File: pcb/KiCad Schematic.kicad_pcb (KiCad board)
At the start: 2 copper layers, 50.1 x 70 mm, 98 parts, among them IC1 AP63205WU-7, IC2 ATSAMD51J19A-MU, J1 47571-0001, J10 Conn_01x04, J11 Conn_01x04, J12 Conn_01x03, J13 Conn_01x03, J14 Conn_01x20, J15 Conn_01x03, J16 Conn_01x03, J17 Hole, J18 Hole, J19 Hole, J2 Conn_01x02, J20 Hole, J21 Conn_01x02, J22 Conn_01x06, J3 47346-0001, J4 Conn_01x04, J5 Conn_01x04, J6 20021121-00010C4LF, J7 Conn_01x02, J8 Conn_01x02, J9 Conn_01x02, Q1 NVTFS5C680NLTAG, Q2 NVTFS5C680NLTAG, U1 TMC2041-LA, U2 TMC2041-LA, U3 AP2112K-3.3, Y1 LFXTAL009678REEL

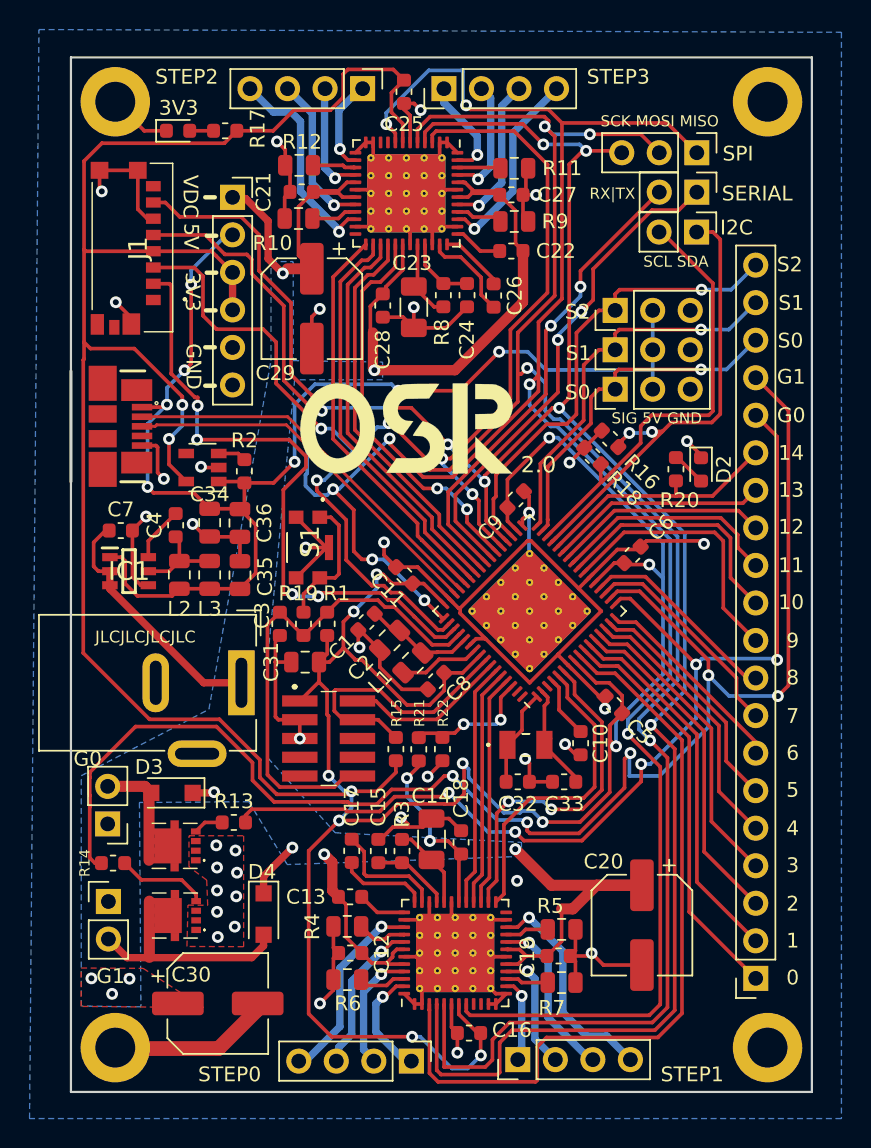
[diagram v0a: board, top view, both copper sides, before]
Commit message: arduino version bump
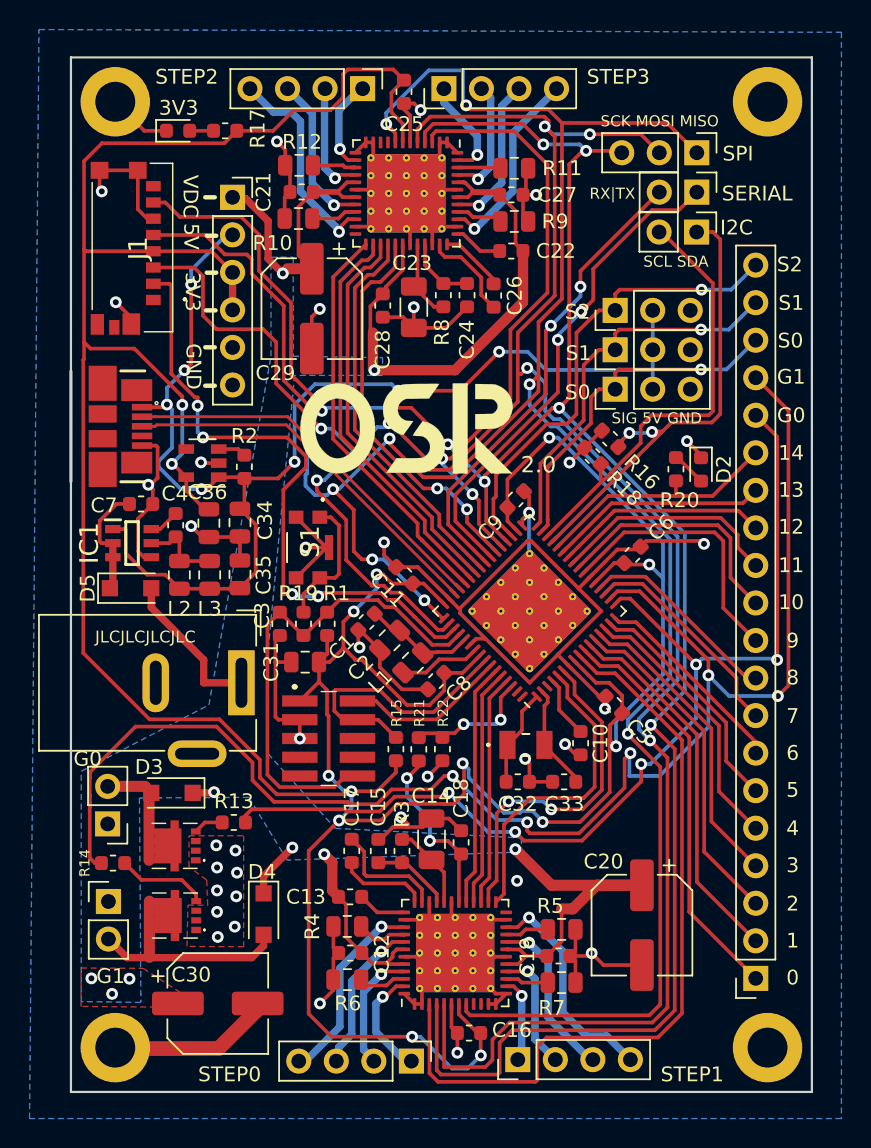
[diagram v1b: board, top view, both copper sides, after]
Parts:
- added D5: CGRTS4004-HF, Diode_SMD:D_SOD-123F, F.Cu at (22.9, 161.8)
- moved C7 2.27 mm to (23.6, 156.1)
- moved C36 2.10 mm to (28.2, 157.4)
- moved C34 2.05 mm to (30.3, 157.4)
- moved IC1 1.91 mm to (23.0, 158.8)
- moved R2 0.30 mm to (30.6, 153.6)
- moved U3 0.30 mm to (27.8, 153.3)
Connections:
- C36 pad 1: +5V -> +3V3
- C7 pad 1: +VDC -> Net-(C7-Pad1)
- IC1 pad 2: +VDC -> Net-(C7-Pad1)
- IC1 pad 3: +VDC -> Net-(C7-Pad1)
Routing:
- net Net-(C7-Pad1): track 0.00 -> 7.96 mm
- net +VDC: track 125.8 -> 119.2 mm
- net +5V: track 88.8 -> 85.4 mm
- net +3V3: track 273.4 -> 276.3 mm
- net Net-(C4-Pad2): track 3.72 -> 2.08 mm
- net GND: track 211.8 -> 213.2 mm, vias 36 -> 35
- net Net-(C4-Pad1): track 6.18 -> 5.62 mm
